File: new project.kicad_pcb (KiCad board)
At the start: 2 copper layers, 44.9 x 35 mm, 4 parts, among them J1 LED 0.170amps, J2 Tractive Battery

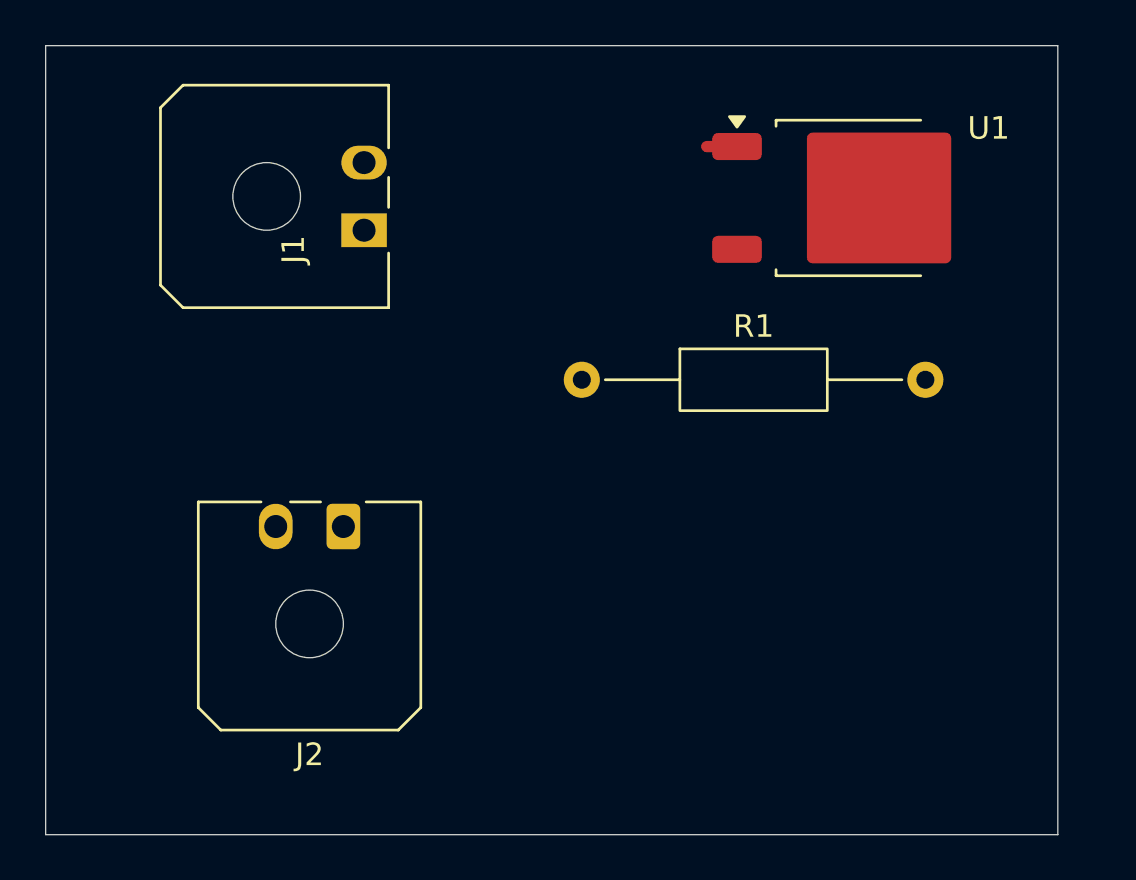
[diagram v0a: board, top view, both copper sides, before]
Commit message: FInished
Done
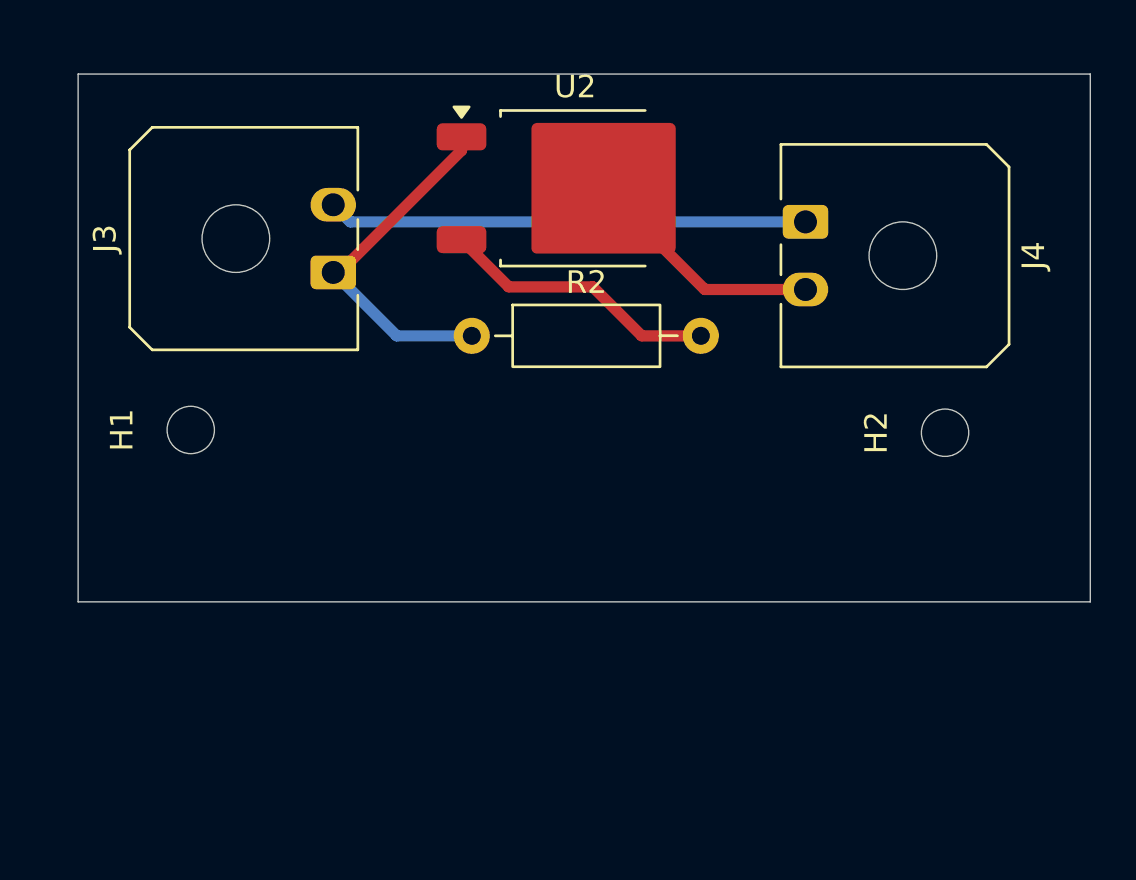
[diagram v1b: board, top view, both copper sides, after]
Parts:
- removed J1: LED 0.170amps, Connector_Molex:Molex_Micro-Fit_3.0_43650-0200_1x02_P3.00mm_Horizontal
- removed J2: Tractive Battery, Connector_Molex:Molex_Micro-Fit_3.0_43650-0200_1x02_P3.00mm_Horizontal
- removed R1: 18000, Resistor_THT:R_Axial_DIN0207_L6.3mm_D2.5mm_P15.24mm_Horizontal
- removed U1: ~, Package_TO_SOT_SMD:TO-252-2
- added H1: MountingHole, MountingHole:MountingHole_2.1mm, F.Cu at (110.6, 75.7)
- added H2: MountingHole, MountingHole:MountingHole_2.1mm, F.Cu at (144.1, 75.8)
- added J3: Tractive Battery, Connector_Molex:Molex_Micro-Fit_3.0_43650-0200_1x02_P3.00mm_Horizontal, F.Cu at (116.9, 68.7)
- added J4: LED 0.170amps, Connector_Molex:Molex_Micro-Fit_3.0_43650-0200_1x02_P3.00mm_Horizontal, F.Cu at (137.9, 66.5)
- added R2: 18000, Resistor_THT:R_Axial_DIN0207_L6.3mm_D2.5mm_P10.16mm_Horizontal, F.Cu at (123.1, 71.6)
- added U2: ~, Package_TO_SOT_SMD:TO-252-2, F.Cu at (127.7, 65.0)
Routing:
- net Net-(J3-Pin_2): track 0.00 -> 21.3 mm
- net GND: track 1.71 -> 16.3 mm
- net Net-(U2-Cathode): track 0.00 -> 12.4 mm
- net Net-(J4-Pin_2): track 0.00 -> 10.8 mm
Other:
- board size 44.9 x 35 mm -> 44.9 x 23.4 mm
